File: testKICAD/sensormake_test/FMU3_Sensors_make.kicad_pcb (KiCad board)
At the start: 2 copper layers, 19.8 x 16 mm, 14 parts, among them J1 Conn_01x06_Male, J2 Conn_01x05, U1 MPU-9250, U2 MS561101BA03-50, U3 ICM-20602

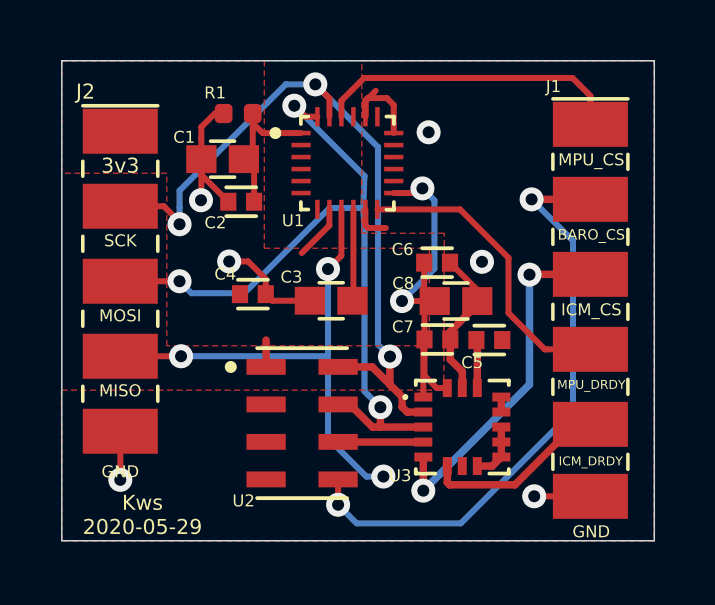
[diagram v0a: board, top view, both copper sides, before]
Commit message: save sensor
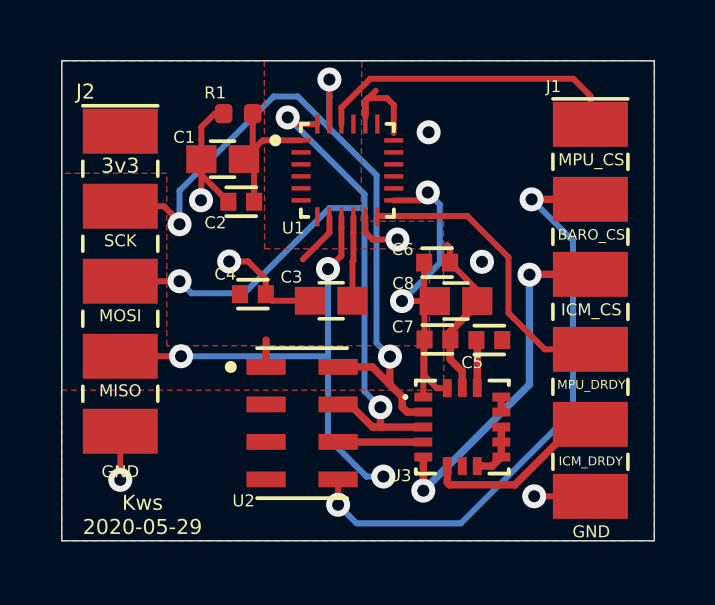
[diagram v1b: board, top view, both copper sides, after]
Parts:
- moved U1 0.24 mm to (138.8, 25.7)
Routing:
- net GND: track 24.5 -> 25.6 mm, vias 6 -> 7
- net /SPI_INT_SCK: track 25.4 -> 26.3 mm
- net /VDD_3V3_SENSORS: track 21.4 -> 21.9 mm
